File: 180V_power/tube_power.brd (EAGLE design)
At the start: 50 x 27 mm, 26 parts, among them IC1 NE555D, Q1 IRF740S, U1 TLV1117-5SOT-223, U2 BC817

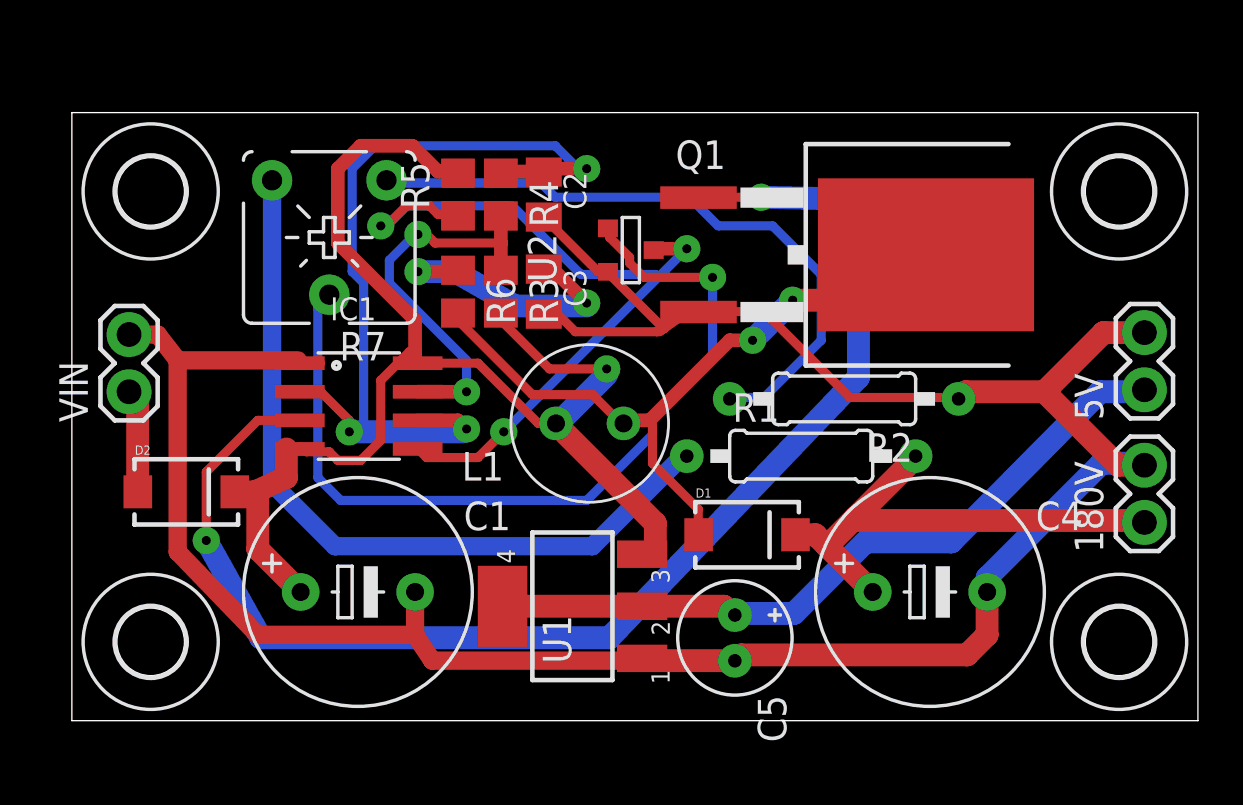
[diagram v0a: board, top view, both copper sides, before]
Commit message: lalala
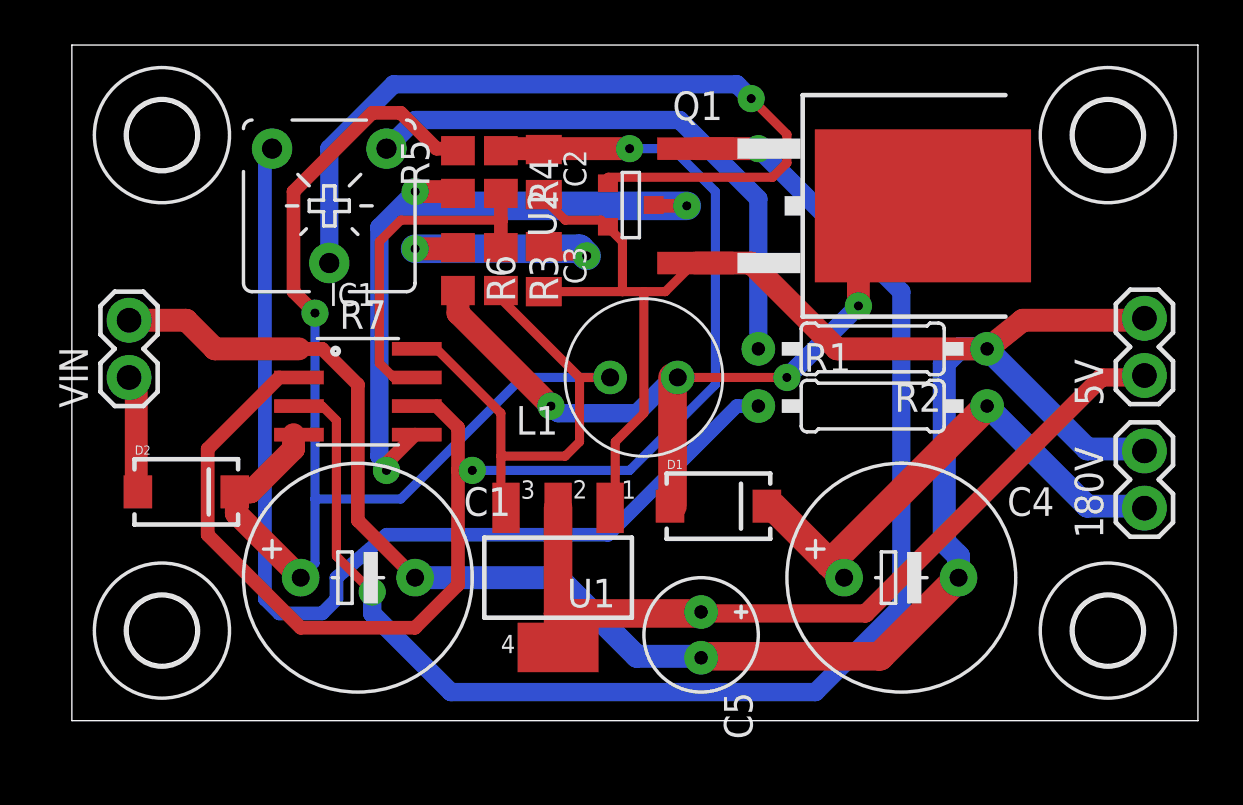
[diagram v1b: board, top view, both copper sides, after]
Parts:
- moved R1 3.88 mm to (35.6, 14.0)
- moved L1 3.15 mm to (25.4, 15.2)
- moved R2 2.56 mm to (35.6, 16.5)
- moved U$1 2.55 mm to (4.00, 26.0)
- moved U$5 2.55 mm to (46.0, 26.0)
- moved Q1 2.18 mm to (34.3, 22.9)
- moved U2 2.00 mm to (24.8, 22.9)
- moved D1 1.80 mm to (28.7, 9.53)
- moved C5 1.51 mm to (27.9, 3.81)
- moved C4 1.42 mm to (36.8, 6.35)
- moved U1 1.42 mm to (21.6, 6.35), turned to 180 degrees
- moved R7 1.41 mm to (11.4, 22.9)
- moved C2 1.00 mm to (21.0, 24.4)
- moved C3 1.00 mm to (21.0, 20.1)
- moved R3 1.00 mm to (19.1, 20.1)
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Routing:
- net THR: track 38.0 -> 64.0 mm, vias 3 -> 2
- net VCC: track 59.6 -> 74.5 mm
- net R1: track 34.7 -> 46.6 mm
- net OUT: track 58.8 -> 63.4 mm
- net CON: track 35.5 -> 31.2 mm
- net R2: track 29.2 -> 25.2 mm
- net 5V: track 32.8 -> 36.7 mm
- net DIS: track 17.4 -> 15.5 mm, vias 2 -> 0
- net VAR: track 38.8 -> 37.2 mm
- net L1: track 35.6 -> 34.3 mm, vias 2 -> 3
- net GND: track 114.2 -> 115.2 mm
- net N$1: track 4.61 -> 5.28 mm
- net R6: track 12.5 -> 11.8 mm
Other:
- board size 50 x 27 mm -> 50 x 30 mm
- board text added: "B"
- board text added: "NIXIE POWER SUPPLY"
- board text added: "oy"
- board text added: "uzz"
